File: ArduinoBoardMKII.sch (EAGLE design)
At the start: 29 parts

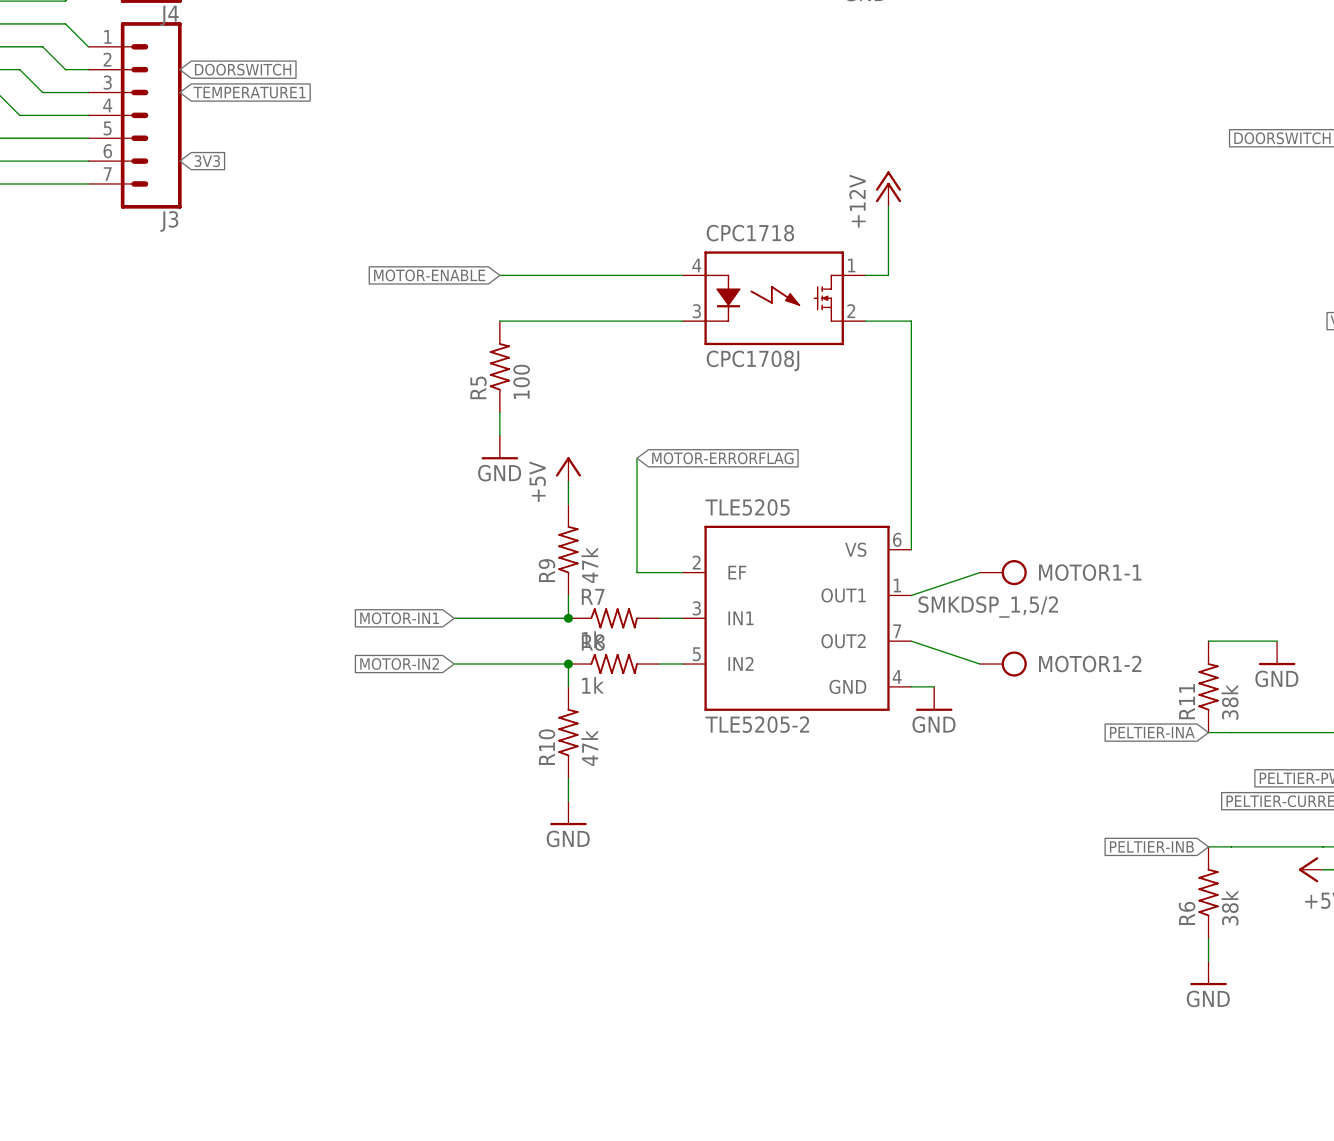
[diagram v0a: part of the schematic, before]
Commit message: Update
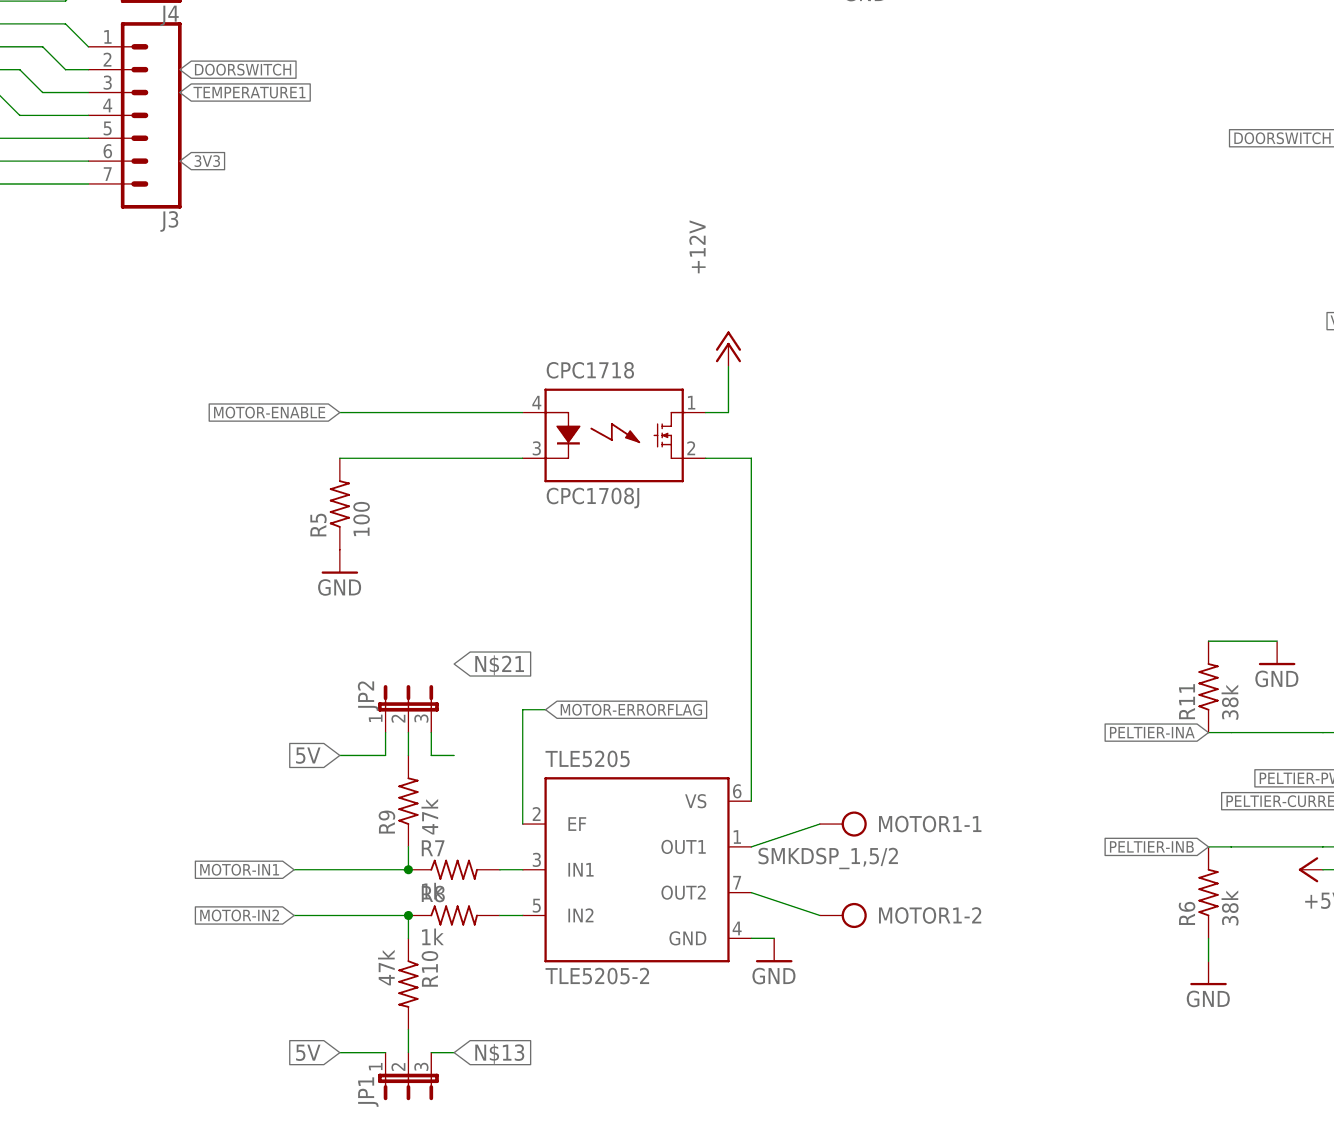
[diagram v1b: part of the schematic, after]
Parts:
- added JP1, JP2: (no value), jumper:JP2E
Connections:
- new net 5V: JP1.1, JP2.1
- new net N$12: JP2.2, R9.2
- new net N$13: JP1.3
- new net N$21: JP2.3
- new net N$4: JP1.2, R10.2
- net +5V: no longer R9.2
- net GND: no longer R10.1
- net MOTOR-IN2: now also R10.1; no longer R10.2
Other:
- moved on the sheet: CPC1718, MOTOR1-1, MOTOR1-2, R10, R5, R7, R8, R9, TLE5205
